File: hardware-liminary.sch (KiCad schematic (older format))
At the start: 2 parts, among them J1 Conn_01x05, J2 Conn_01x05

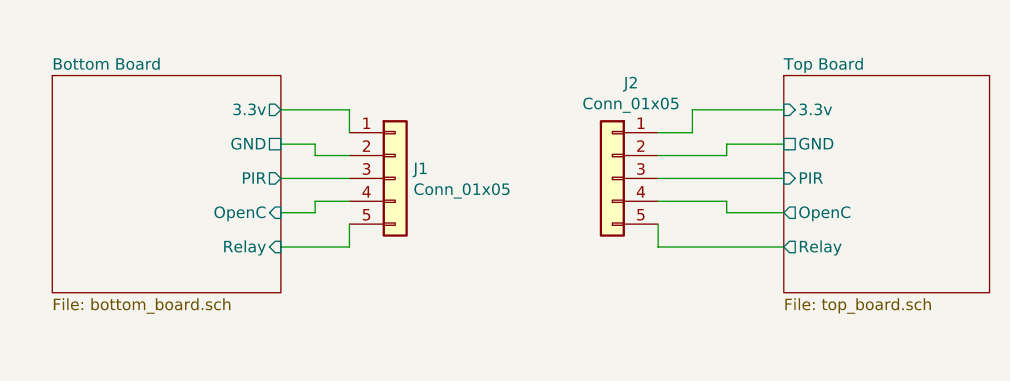
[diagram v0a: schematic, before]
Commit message: Agregado modulo HLW8032
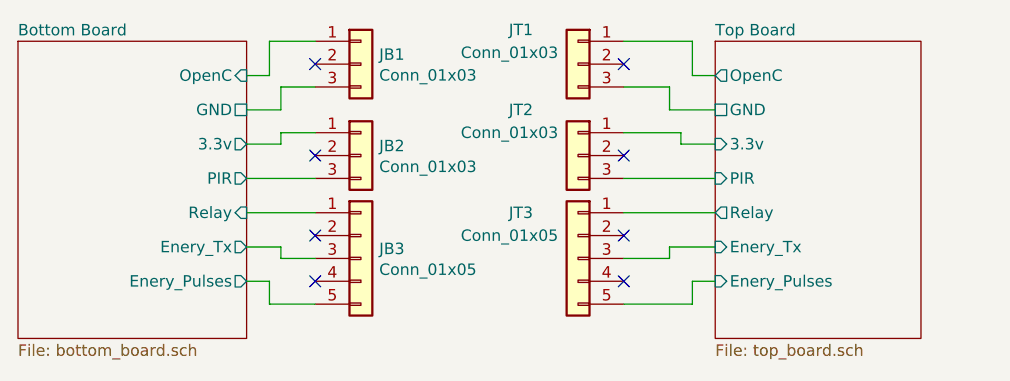
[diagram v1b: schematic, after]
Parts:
- removed J1, J2: Conn_01x05, Connector_PinHeader_2.54mm:PinHeader_1x05_P2.54mm_Vertical, symbol Connector_Generic:Conn_01x05
- added JB1, JB2, JT1, JT2: Conn_01x03, Connector_PinHeader_2.54mm:PinHeader_1x03_P2.54mm_Vertical, symbol Connector_Generic:Conn_01x03
- added JB3, JT3: Conn_01x05, Connector_PinHeader_2.54mm:PinHeader_1x05_P2.54mm_Vertical, symbol Connector_Generic:Conn_01x05
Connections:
- net Bottom Board/3.3v: now also JB2.1 (Pin_1)
- net Bottom Board/GND: now also JB1.3 (Pin_3)
- net Bottom Board/OpenC: now also JB1.1 (Pin_1)
- net Bottom Board/PIR: now also JB2.3 (Pin_3)
- net Bottom Board/Relay: now also JB3.1 (Pin_1)
- net Top Board/3.3v: now also JT2.1 (Pin_1)
- net Top Board/GND: now also JT1.3 (Pin_3)
- net Top Board/OpenC: now also JT1.1 (Pin_1)
- net Top Board/PIR: now also JT2.3 (Pin_3)
- net Top Board/Relay: now also JT3.1 (Pin_1)
- new net Bottom Board/Enery_Pulses: JB3.5 (Pin_5)
- new net Bottom Board/Enery_Tx: JB3.3 (Pin_3)
- new net Top Board/Enery_Pulses: JT3.5 (Pin_5)
- new net Top Board/Enery_Tx: JT3.3 (Pin_3)
- no-connect marks 0 -> 8
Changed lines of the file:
@@
 $EndDescr
 $Sheet
-S 5550 3150 900  950
+S 5250 3000 900  1300
 U 5F84ED08
 F0 "Top Board" 50
 F1 "top_board.sch" 50
-F2 "3.3v" I L 5550 3300 50
-F3 "GND" U L 5550 3450 50
-F4 "OpenC" O L 5550 3750 50
-F5 "PIR" I L 5550 3600 50
-F6 "Relay" O L 5550 3900 50
+F2 "3.3v" I L 5250 3450 50
+F3 "GND" U L 5250 3300 50
+F4 "OpenC" O L 5250 3150 50
+F5 "PIR" I L 5250 3600 50
+F6 "Relay" O L 5250 3750 50
+F7 "Enery_Tx" I L 5250 3900 50
+F8 "Enery_Pulses" I L 5250 4050 50
 $EndSheet
 $Sheet
-S 2350 3150 1000 950
+S 2200 3000 1000 1300
 U 5F91F411
 F0 "Bottom Board" 50
 F1 "bottom_board.sch" 50
-F2 "3.3v" O R 3350 3300 50
-F3 "GND" U R 3350 3450 50
-F4 "OpenC" I R 3350 3750 50
-F5 "PIR" O R 3350 3600 50
-F6 "Relay" I R 3350 3900 50
+F2 "3.3v" O R 3200 3450 50
+F3 "GND" U R 3200 3300 50
+F4 "OpenC" I R 3200 3150 50
+F5 "PIR" O R 3200 3600 50
+F6 "Relay" I R 3200 3750 50
+F7 "Enery_Tx" O R 3200 3900 50
+F8 "Enery_Pulses" O R 3200 4050 50
 $EndSheet
 $Comp
-L Connector_Generic:Conn_01x05 J1
-U 1 1 5F94C7D4
-P 3850 3600
-F 0 "J1" H 3930 3642 50  0000 L CNN
-F 1 "Conn_01x05" H 3930 3551 50  0000 L CNN
-F 2 "Connector_PinHeader_2.54mm:PinHeader_1x05_P2.54mm_Vertical" H 3850 3600 50  0001 C CNN
-F 3 "~" H 3850 3600 50  0001 C CNN
-	1    3850 3600
+L Connector_Generic:Conn_01x03 JB1
+U 1 1 5F8428AB
+P 3700 3100
+F 0 "JB1" H 3780 3142 50  0000 L CNN
+F 1 "Conn_01x03" H 3780 3051 50  0000 L CNN
+F 2 "Connector_PinHeader_2.54mm:PinHeader_1x03_P2.54mm_Vertical" H 3700 3100 50  0001 C CNN
+F 3 "~" H 3700 3100 50  0001 C CNN
+	1    3700 3100
 	1    0    0    -1
 $EndComp
 $Comp
-L Connector_Generic:Conn_01x05 J2
-U 1 1 5F94DC5D
-P 4800 3600
-F 0 "J2" H 4718 4017 50  0000 C CNN
-F 1 "Conn_01x05" H 4718 3926 50  0000 C CNN
-F 2 "Connector_PinHeader_2.54mm:PinHeader_1x05_P2.54mm_Vertical" H 4800 3600 50  0001 C CNN
-F 3 "~" H 4800 3600 50  0001 C CNN
-	1    4800 3600
+L Connector_Generic:Conn_01x03 JT1
+U 1 1 5F844220
+P 4650 3100
+F 0 "JT1" H 4900 3250 50  0000 C CNN
+F 1 "Conn_01x03" H 4950 3150 50  0000 C CNN
+F 2 "Connector_PinHeader_2.54mm:PinHeader_1x03_P2.54mm_Vertical" H 4650 3100 50  0001 C CNN
+F 3 "~" H 4650 3100 50  0001 C CNN
+	1    4650 3100
+	-1   0    0    -1
+$EndComp
+NoConn ~ 3500 3100
+NoConn ~ 4850 3100
+Wire Wire Line
+	3200 3150 3300 3150
+Wire Wire Line
+	3300 3150 3300 3000
+Wire Wire Line
+	3300 3000 3500 3000
+Wire Wire Line
+	3200 3300 3350 3300
+Wire Wire Line
+	3350 3300 3350 3200
+Wire Wire Line
+	3350 3200 3500 3200
+Wire Wire Line
+	5250 3300 5050 3300
+Wire Wire Line
+	5050 3300 5050 3200
+Wire Wire Line
+	5050 3200 4850 3200
+Wire Wire Line
+	5250 3150 5150 3150
+Wire Wire Line
+	5150 3150 5150 3000
+Wire Wire Line
+	5150 3000 4850 3000
+$Comp
+L Connector_Generic:Conn_01x03 JB2
+U 1 1 5F84642D
+P 3700 3500
+F 0 "JB2" H 3780 3542 50  0000 L CNN
+F 1 "Conn_01x03" H 3780 3451 50  0000 L CNN
+F 2 "Connector_PinHeader_2.54mm:PinHeader_1x03_P2.54mm_Vertical" H 3700 3500 50  0001 C CNN
+F 3 "~" H 3700 3500 50  0001 C CNN
+	1    3700 3500
+	1    0    0    -1
+$EndComp
+$Comp
+L Connector_Generic:Conn_01x03 JT2
+U 1 1 5F846D28
+P 4650 3500
+F 0 "JT2" H 4900 3700 50  0000 C CNN
+F 1 "Conn_01x03" H 4950 3600 50  0000 C CNN
+F 2 "Connector_PinHeader_2.54mm:PinHeader_1x03_P2.54mm_Vertical" H 4650 3500 50  0001 C CNN
+F 3 "~" H 4650 3500 50  0001 C CNN
+	1    4650 3500
 	-1   0    0    -1
 $EndComp
 Wire Wire Line
-	3350 3300 3650 3300
+	3200 3600 3500 3600
 Wire Wire Line
-	3650 3300 3650 3400
+	3200 3450 3350 3450
 Wire Wire Line
-	3350 3450 3500 3450
+	3350 3450 3350 3400
 Wire Wire Line
-	3500 3450 3500 3500
+	3350 3400 3500 3400
 Wire Wire Line
-	3500 3500 3650 3500
+	4850 3600 5250 3600
 Wire Wire Line
-	3350 3600 3650 3600
+	5250 3450 5100 3450
 Wire Wire Line
-	3350 3750 3500 3750
+	5100 3450 5100 3400
 Wire Wire Line
-	3500 3750 3500 3700
+	5100 3400 4850 3400
+NoConn ~ 4850 3500
+NoConn ~ 3500 3500
+$Comp
+L Connector_Generic:Conn_01x05 JB3
+U 1 1 5F84843D
+P 3700 3950
+F 0 "JB3" H 3780 3992 50  0000 L CNN
+F 1 "Conn_01x05" H 3780 3901 50  0000 L CNN
+F 2 "Connector_PinHeader_2.54mm:PinHeader_1x05_P2.54mm_Vertical" H 3700 3950 50  0001 C CNN
+F 3 "~" H 3700 3950 50  0001 C CNN
+	1    3700 3950
+	1    0    0    -1
+$EndComp
+$Comp
+L Connector_Generic:Conn_01x05 JT3
+U 1 1 5F84914E
+P 4650 3950
+F 0 "JT3" H 4900 4150 50  0000 C CNN
+F 1 "Conn_01x05" H 4950 4050 50  0000 C CNN
+F 2 "Connector_PinHeader_2.54mm:PinHeader_1x05_P2.54mm_Vertical" H 4650 3950 50  0001 C CNN
+F 3 "~" H 4650 3950 50  0001 C CNN
+	1    4650 3950
+	-1   0    0    -1
+$EndComp
 Wire Wire Line
-	3500 3700 3650 3700
+	3200 3750 3500 3750
 Wire Wire Line
-	3350 3900 3650 3900
+	3200 3900 3350 3900
 Wire Wire Line
-	3650 3900 3650 3800
+	3350 3900 3350 3950
 Wire Wire Line
-	5000 3600 5550 3600
+	3350 3950 3500 3950
 Wire Wire Line
-	5000 3500 5300 3500
+	3200 4050 3300 4050
 Wire Wire Line
-	5300 3500 5300 3450
+	3300 4050 3300 4150
 Wire Wire Line
-	5300 3450 5550 3450
+	3300 4150 3500 4150
 Wire Wire Line
-	5000 3800 5000 3900
+	5250 3750 4850 3750
 Wire Wire Line
-	5000 3900 5550 3900
+	5250 3900 5050 3900
 Wire Wire Line
-	5550 3750 5300 3750
+	5050 3900 5050 3950
 Wire Wire Line
-	5300 3750 5300 3700
+	5050 3950 4850 3950
 Wire Wire Line
-	5300 3700 5000 3700
+	5250 4050 5150 4050
 Wire Wire Line
-	5000 3400 5150 3400
+	5150 4050 5150 4150
 Wire Wire Line
-	5150 3400 5150 3300
-Wire Wire Line
-	5150 3300 5550 3300
+	5150 4150 4850 4150
+NoConn ~ 3500 3850
+NoConn ~ 3500 4050
+NoConn ~ 4850 3850
+NoConn ~ 4850 4050
 $EndSCHEMATC
